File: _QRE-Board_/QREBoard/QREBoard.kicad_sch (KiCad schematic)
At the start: 11 parts, among them J1 Conn_01x04_Pin

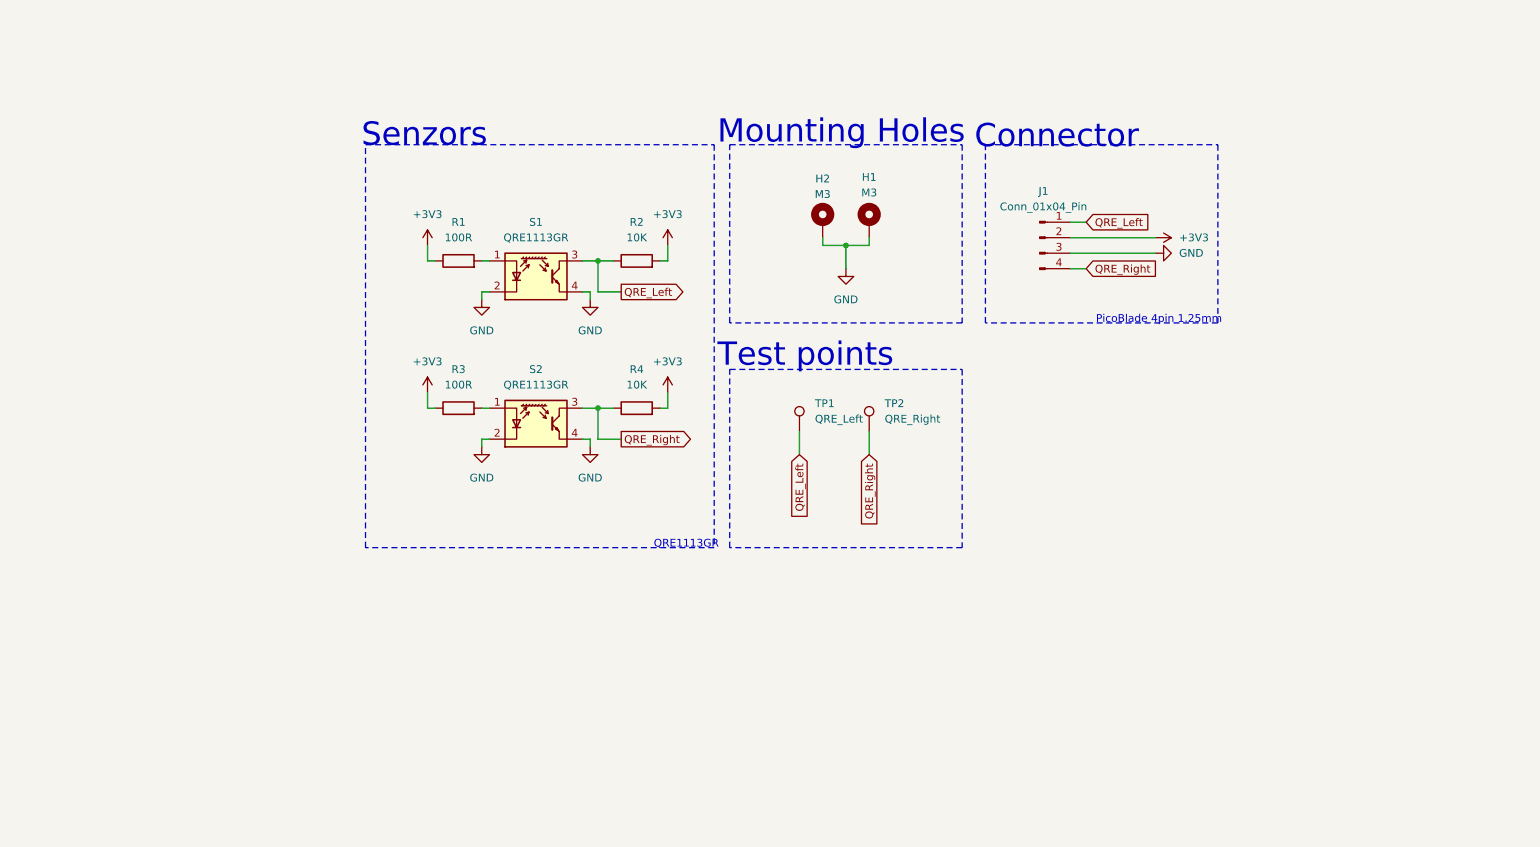
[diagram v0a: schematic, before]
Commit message: some changes
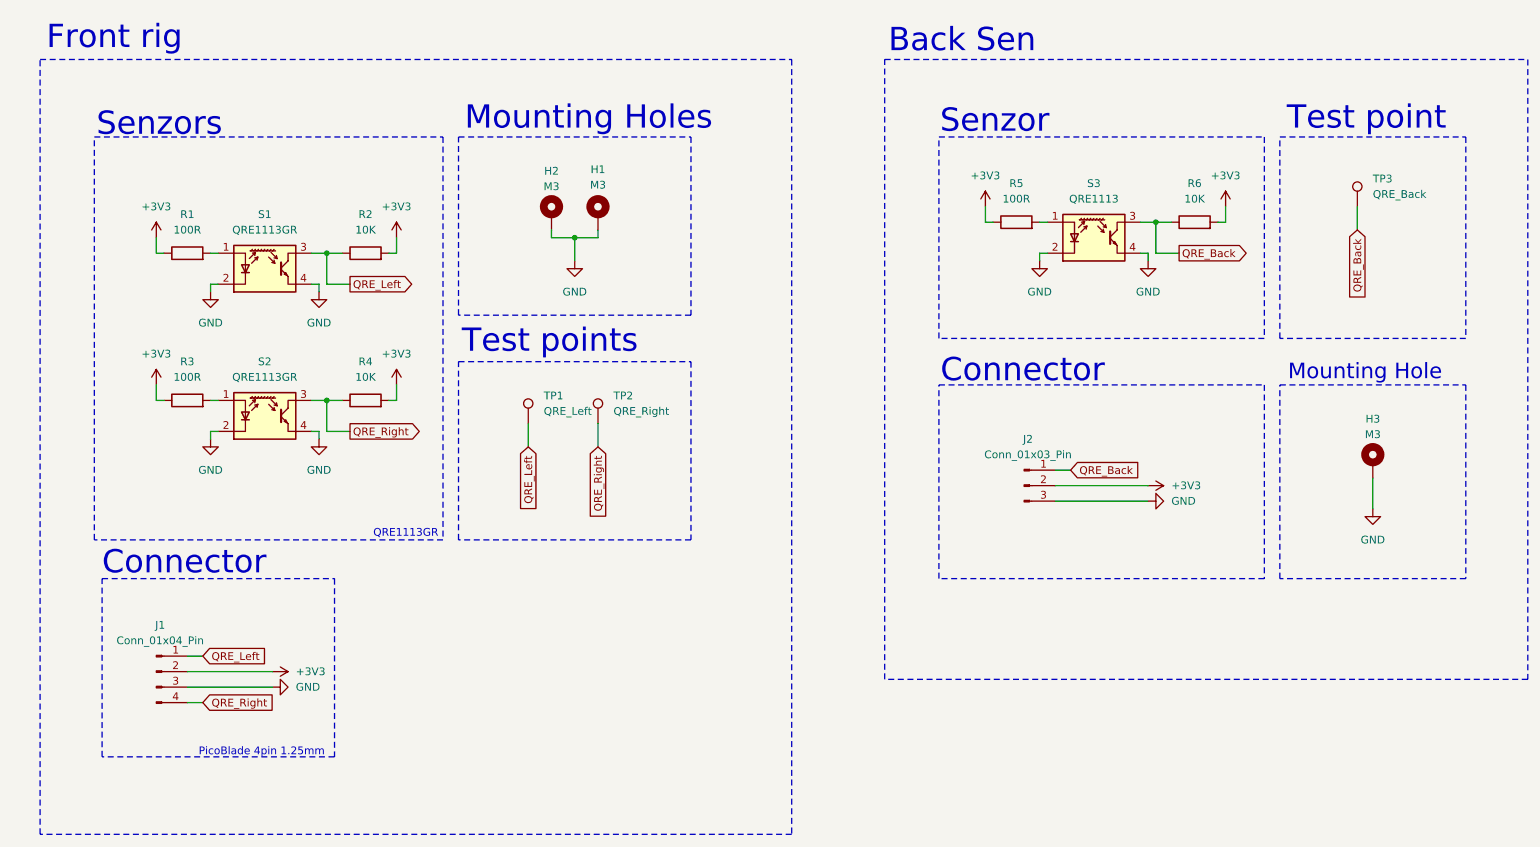
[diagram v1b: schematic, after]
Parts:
- added H3: M3, MountingHole:MountingHole_3.2mm_M3_Pad_Via, symbol Mechanical:MountingHole_Pad
- added J2: Conn_01x03_Pin, Connector:FanPinHeader_1x03_P2.54mm_Vertical, symbol Connector:Conn_01x03_Pin
- added R5: 100R, Resistor_SMD:R_0805_2012Metric_Pad1.20x1.40mm_HandSolder, symbol Device:R
- added R6: 10K, Resistor_SMD:R_0805_2012Metric_Pad1.20x1.40mm_HandSolder, symbol Device:R
- added S3: QRE1113, OptoDevice:OnSemi_CASE100AQ, symbol Sensor_Proximity:QRE1113
- added TP3: QRE_Back, TestPoint:TestPoint_Pad_D1.5mm, symbol Connector:TestPoint
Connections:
- net +3V3: now also J2.2 (Pin_2), R5.1, R6.2
- net GND: now also H3.1, J2.3 (Pin_3), S3.2 (K), S3.4
- new net: R5.2, S3.1 (A)
- new net QRE_Back: J2.1 (Pin_1), R6.1, S3.3, TP3.1
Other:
- note added: "Back Sen"
- note added: "Front rig"
- note added: "Mounting Hole"
- note added: "Senzor"
- note added: "Test point"
- moved on the sheet: H1, H2, J1, R1, R2, R3, R4, S1, S2, TP1, TP2

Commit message: QRE-BOARD UPDATE
Redesighned QRE-BackSen to maxbe latest eteration for now

Added some changes on mk-1 DPS desighn too (Not that much)
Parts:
- H3: footprint MountingHole:MountingHole_3.2mm_M3_Pad_Via -> MountingHole:MountingHole_3.2mm_M3_ISO7380_Pad_TopBottom
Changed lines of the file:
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@@
 			)
 		)
-		(property "Footprint" "MountingHole:MountingHole_3.2mm_M3_Pad_Via"
+		(property "Footprint" "MountingHole:MountingHole_3.2mm_M3_ISO7380_Pad_TopBottom"
 			(at 246.38 100.33 0)
 			(hide yes)
